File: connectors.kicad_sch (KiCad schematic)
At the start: 6 parts, among them J1 Conn_01x05, J2 Conn_01x07, J3 Conn_01x01, J4 Conn_01x07, J5 HW-769, J7 Conn_01x03

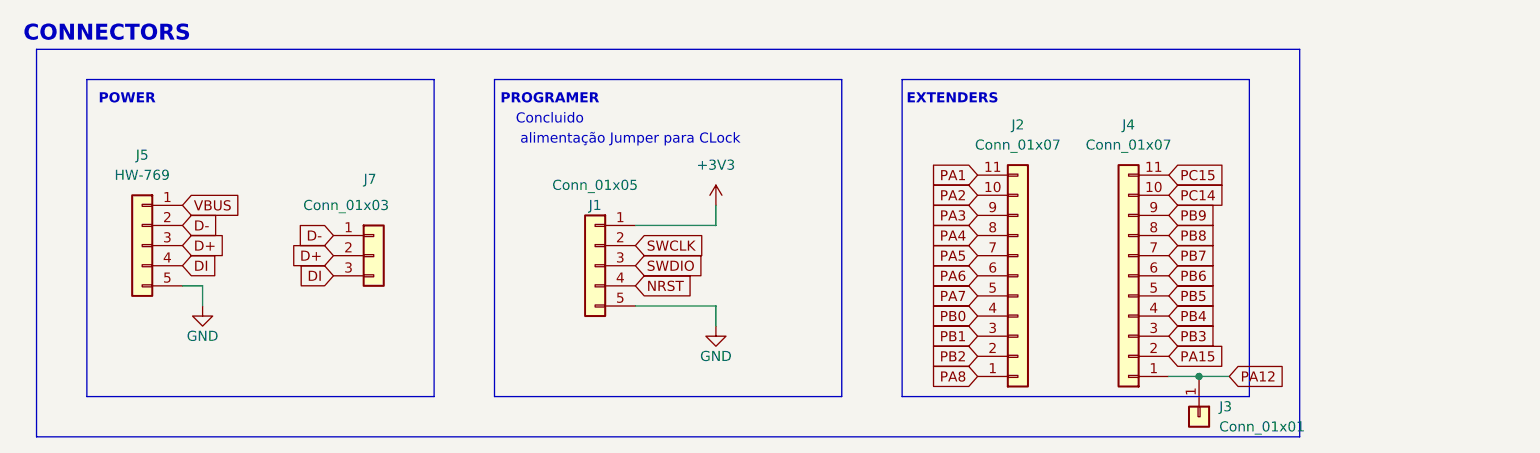
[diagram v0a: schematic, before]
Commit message: perf: 45° micro
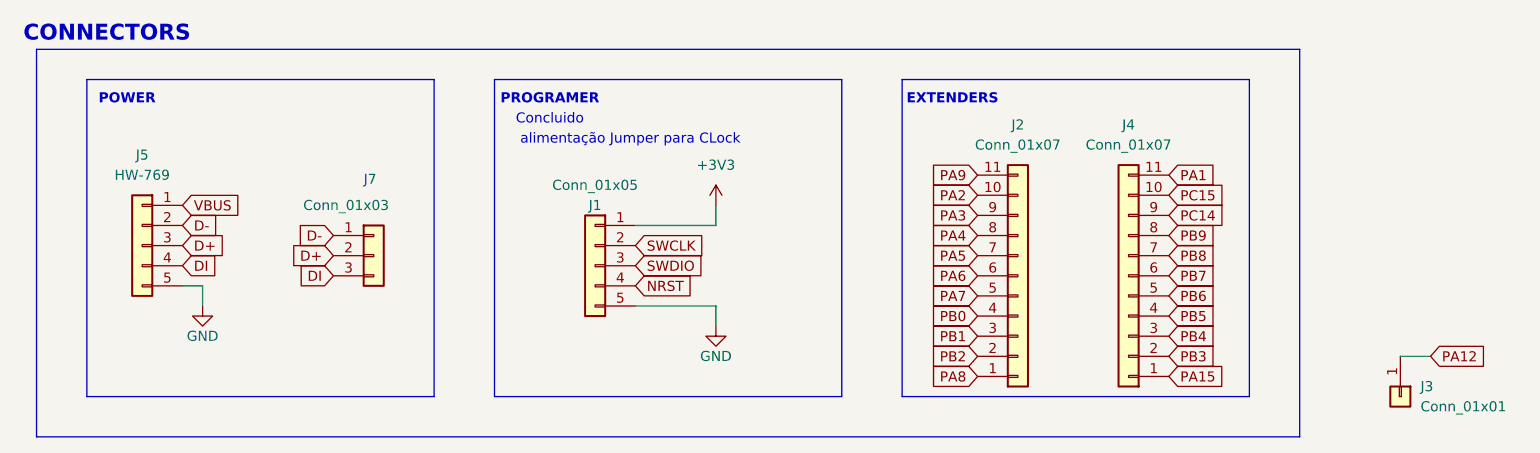
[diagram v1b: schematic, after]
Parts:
- J3: footprint TestPoint:TestPoint_THTPad_1.0x1.0mm_Drill0.5mm -> TestPoint_THTPad_D2.0mm_Drill1.0mm
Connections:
- net PA1: now also J4.11 (Pin_11); no longer J2.11 (Pin_11)
- net PA12: no longer J4.1 (Pin_1)
- net PA15: now also J4.1 (Pin_1); no longer J4.2 (Pin_2)
- net PB3: now also J4.2 (Pin_2); no longer J4.3 (Pin_3)
- net PB4: now also J4.3 (Pin_3); no longer J4.4 (Pin_4)
- net PB5: now also J4.4 (Pin_4); no longer J4.5 (Pin_5)
- net PB6: now also J4.5 (Pin_5); no longer J4.6 (Pin_6)
- net PB7: now also J4.6 (Pin_6); no longer J4.7 (Pin_7)
- net PB8: now also J4.7 (Pin_7); no longer J4.8 (Pin_8)
- net PB9: now also J4.8 (Pin_8); no longer J4.9 (Pin_9)
- net PC14: now also J4.9 (Pin_9); no longer J4.10 (Pin_10)
- net PC15: now also J4.10 (Pin_10); no longer J4.11 (Pin_11)
- new net PA9: J2.11 (Pin_11)
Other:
- moved on the sheet: J3

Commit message: board v1
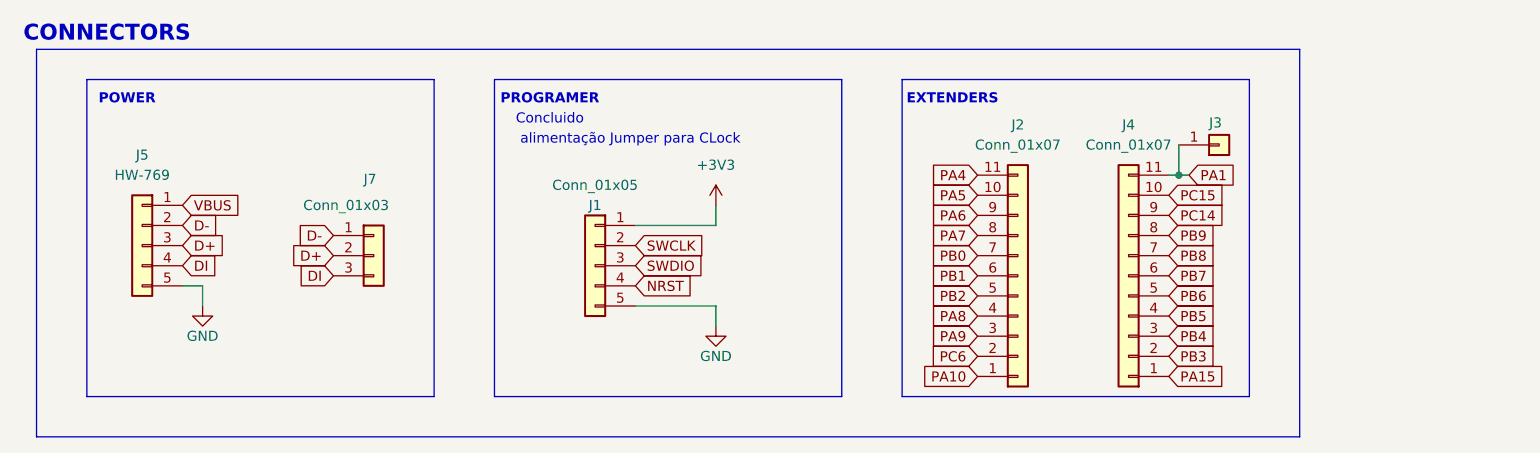
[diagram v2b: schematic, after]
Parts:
- J3: footprint TestPoint_THTPad_D2.0mm_Drill1.0mm -> personalized:hole
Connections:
- net PA12 is gone; now on net PA1: J3.1 (Pin_1)
- net PA2 is gone; now on net PA5: J2.10 (Pin_10)
- net PA3 is gone; now on net PA6: J2.9 (Pin_9)
- net PA4: now also J2.11 (Pin_11); no longer J2.8 (Pin_8)
- net PA5: no longer J2.7 (Pin_7)
- net PA6: no longer J2.6 (Pin_6)
- net PA7: now also J2.8 (Pin_8); no longer J2.5 (Pin_5)
- net PA8: now also J2.4 (Pin_4); no longer J2.1 (Pin_1)
- net PA9: now also J2.3 (Pin_3); no longer J2.11 (Pin_11)
- net PB0: now also J2.7 (Pin_7); no longer J2.4 (Pin_4)
- net PB1: now also J2.6 (Pin_6); no longer J2.3 (Pin_3)
- net PB2: now also J2.5 (Pin_5); no longer J2.2 (Pin_2)
- new net PA10: J2.1 (Pin_1)
- new net PC6: J2.2 (Pin_2)
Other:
- moved on the sheet: J3
